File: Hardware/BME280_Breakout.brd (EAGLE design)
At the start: 12.7 x 20.3 mm, 20 parts, among them U1 BME280

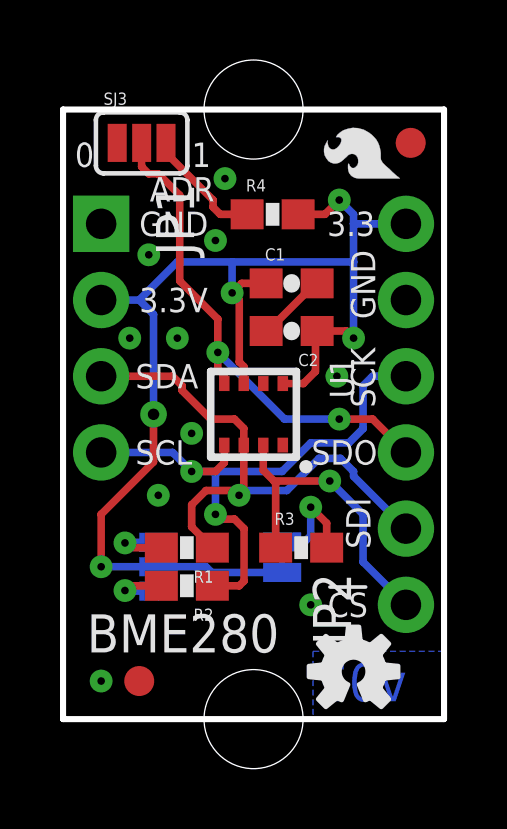
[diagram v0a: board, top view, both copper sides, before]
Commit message: Rev 0.2
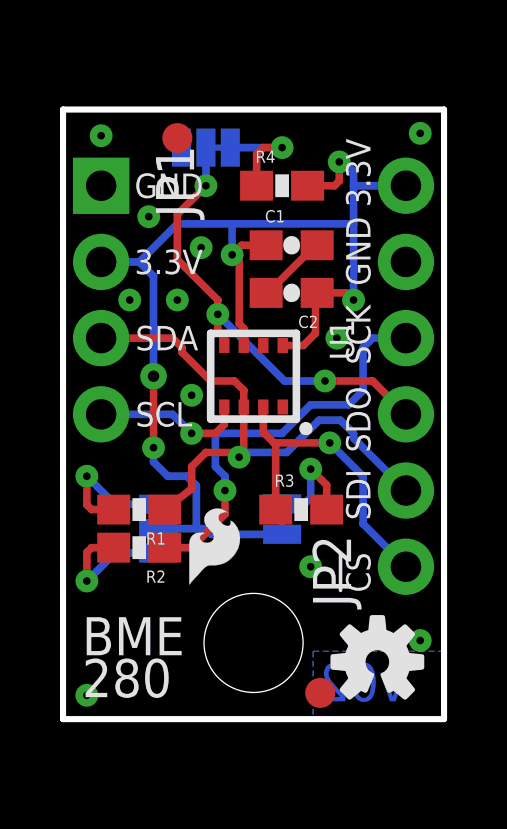
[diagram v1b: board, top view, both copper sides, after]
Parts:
- removed STANDOFF1: STAND-OFF, SparkFun-Electromechanical:STAND-OFF
- LOGO1: value SFE_LOGO_NAME.1_INCH -> SFE_LOGO_FLAME.1_INCH; device SparkFun-Aesthetics:SFE_LOGO_NAME_.1 -> SparkFun-Aesthetics:SFE_LOGO_FLAME_.1
- SJ3: device SparkFun-Passives:PAD-JUMPER-3-2OF3_NC_BY_PASTE_YES_SILK_FULL_BOX -> SparkFun-Passives:PAD-JUMPER-3-2OF3_NC_BY_TRACE_YES_SILK_FULL_BOX
- moved LOGO2 15.6 mm to (3.89, 4.13), turned to 0 degrees
- moved LOGO1 8.33 mm to (7.46, 10.0), turned to 0 degrees
- moved FID1 7.78 mm to (3.81, 19.4)
- moved FID2 6.05 mm to (8.57, 0.87)
- moved STANDOFF4 2.54 mm to (6.35, 2.54)
- moved SJ3 2.15 mm to (4.76, 19.1), flipped to the bottom, turned to 180 degrees
- moved R1 2.03 mm to (2.54, 6.99)
- moved R2 2.03 mm to (2.54, 5.71)
- moved C2 1.27 mm to (7.62, 14.2)
- moved R3 1.27 mm to (7.94, 6.99)
- moved SJ2 1.27 mm to (7.30, 6.67)
- moved JP2 1.27 mm to (11.4, 5.08)
- moved C1 1.27 mm to (7.62, 15.8)
- moved JP1 1.27 mm to (1.27, 17.8)
- moved SJ1 1.27 mm to (3.17, 6.35)
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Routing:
- net N$2: track 2.40 -> 4.68 mm
- net N$1: track 2.40 -> 4.68 mm
- net SDO/ADR: track 17.0 -> 15.4 mm, vias 2 -> 3
- net 3.3V: track 42.4 -> 41.0 mm
- net N$4: track 4.03 -> 3.72 mm, vias 0 -> 1
- net GND: vias 10 -> 11
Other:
- board text added: "ADR:"
- board text added: "BME 280"
- board text added: "ENB P-UP"
- board text added: "v02"
- board text removed: "ADR"
- board text removed: "BME280"
- board text removed: "PULL_EN"
- board text removed: "v01"
